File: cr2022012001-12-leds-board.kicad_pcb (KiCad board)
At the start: 2 copper layers, 79.7 x 67.8 mm, 49 parts, among them J1 USB_B_Micro, J2 Conn_01x04, J3 AVR-ISP-6, SW1 SW_Push, U1 ATtiny85-20PU, U2 ATtiny85-20SU

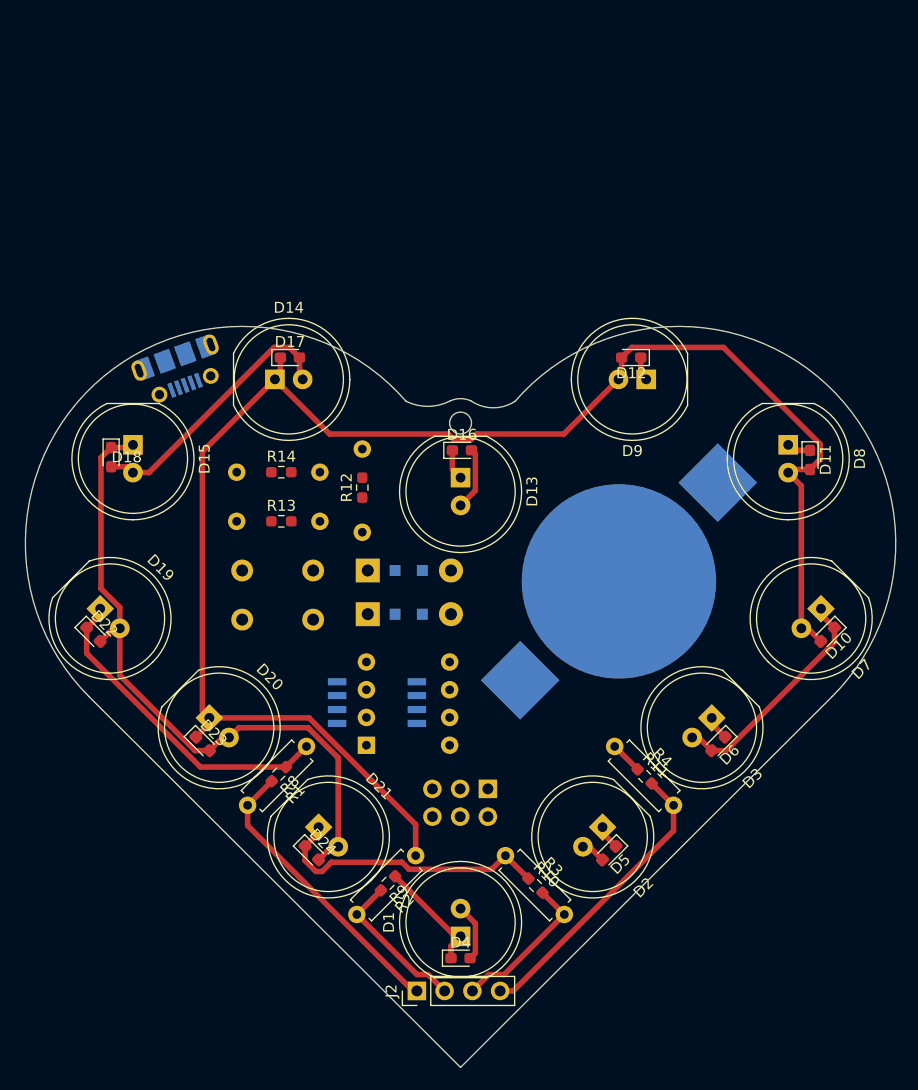
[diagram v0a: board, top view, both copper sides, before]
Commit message: revNC
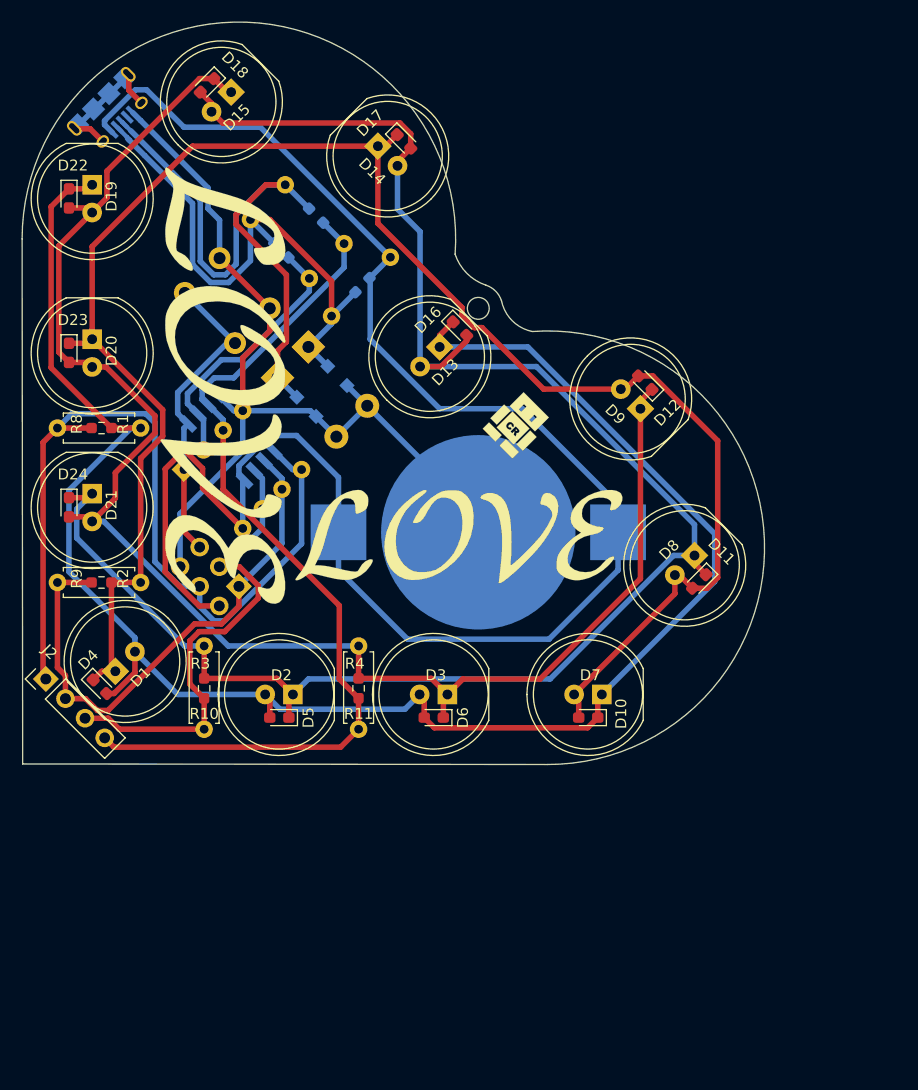
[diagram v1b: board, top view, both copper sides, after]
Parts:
- added G***: LOGO, CAROBOT_KiCad_Footprint:Logo_CAROBOT_Robot_5mm, B.Cu at (159.8, 54.3)
- added G***: LOGO, CAROBOT_KiCad_Footprint:Text_LOVE_9mm, F.Cu at (189.9, 79.4)
- added G***: LOGO, CAROBOT_KiCad_Footprint:Text_LOVE_12mm, F.Cu at (168.3, 65.6)
- added G***: LOGO, CAROBOT_KiCad_Footprint:Logo_CAROBOT_Robot_5mm, F.Cu at (195.2, 69.1)
- J1: footprint Connector_USB:USB_Micro-B_Molex-105017-0001 -> Connector_USB:USB_Micro-B_Amphenol_10118194_Horizontal
- R12, R13, R14: moved to B.Cu
- moved J2 44.4 mm to (152.0, 92.4), turned to 45 degrees
- moved D4 41.3 mm to (157.0, 93.1), turned to 315 degrees
- moved D22 40.0 mm to (154.1, 48.4), turned to 270 degrees
- moved D1 39.9 mm to (158.4, 91.7), turned to 45 degrees
- moved D19 38.8 mm to (156.3, 47.2), turned to 270 degrees
- moved D24 38.7 mm to (154.1, 76.7), turned to 270 degrees
- moved R9 38.0 mm to (157.1, 83.6), turned to 180 degrees
- moved D23 37.8 mm to (154.1, 62.6), turned to 270 degrees
- moved D21 36.9 mm to (156.3, 75.5), turned to 270 degrees
- moved D20 36.3 mm to (156.3, 61.3), turned to 270 degrees
- moved R8 35.6 mm to (157.1, 69.5), turned to 180 degrees
- moved R2 35.5 mm to (160.7, 83.6), turned to 180 degrees
- moved R10 35.3 mm to (166.5, 93.3), turned to 270 degrees
- moved D18 35.2 mm to (166.8, 38.1), turned to 225 degrees
- moved R3 33.6 mm to (166.5, 89.4), turned to 270 degrees
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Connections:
- J1 pad 4: (no net) -> Net-(J1-Pad4)
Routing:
- net VCC: track 0.00 -> 163.0 mm
- net Net-(D1-Pad2): track 61.5 -> 167.7 mm
- net Net-(D11-Pad1): track 61.4 -> 164.6 mm
- net GND: track 0.10 -> 85.1 mm
- net Net-(D12-Pad1): track 69.1 -> 144.6 mm
- net Net-(D26-Pad1): track 0.00 -> 58.6 mm
- net Net-(J2-Pad4): track 27.1 -> 83.7 mm
- net Net-(J2-Pad1): track 26.8 -> 79.0 mm
- net Net-(D25-Pad1): track 0.00 -> 51.5 mm
- net Net-(J2-Pad2): track 14.1 -> 50.0 mm
- net Net-(J2-Pad3): track 14.1 -> 44.3 mm
- net Net-(J3-Pad5): track 0.00 -> 28.9 mm
- net Net-(R13-Pad1): track 0.00 -> 24.6 mm
- net Net-(J1-Pad6): track 0.00 -> 12.0 mm
- net Net-(D1-Pad1): track 157.2 -> 165.2 mm
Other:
- board size 79.7 x 67.8 mm -> 68 x 68 mm
- board text added: "2022-01-21 JKL Rev-NC"
- board text added: "carobot.ca"
